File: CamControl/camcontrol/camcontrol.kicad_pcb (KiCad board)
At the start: 2 copper layers, 35 x 35 mm, 74 parts, among them J2 USB_B_Micro, J3 Conn_01x03, J4 Conn_01x02, J5 Conn_01x02, J6 Conn_01x02, J7 Conn_01x03, J8 Conn_01x04, Q2 AO3401A, Q3 AO3401A, U1 E22-900MM22S, U2 TPS1HC30BQPWPRQ1, U3 TPS63060DSCR, U4 XC6206P332MR, U5 W25Q128JVS, U6 RP2040, U7 TPS1HC30BQPWPRQ1, X1 SX1M12.000M10F30TNN

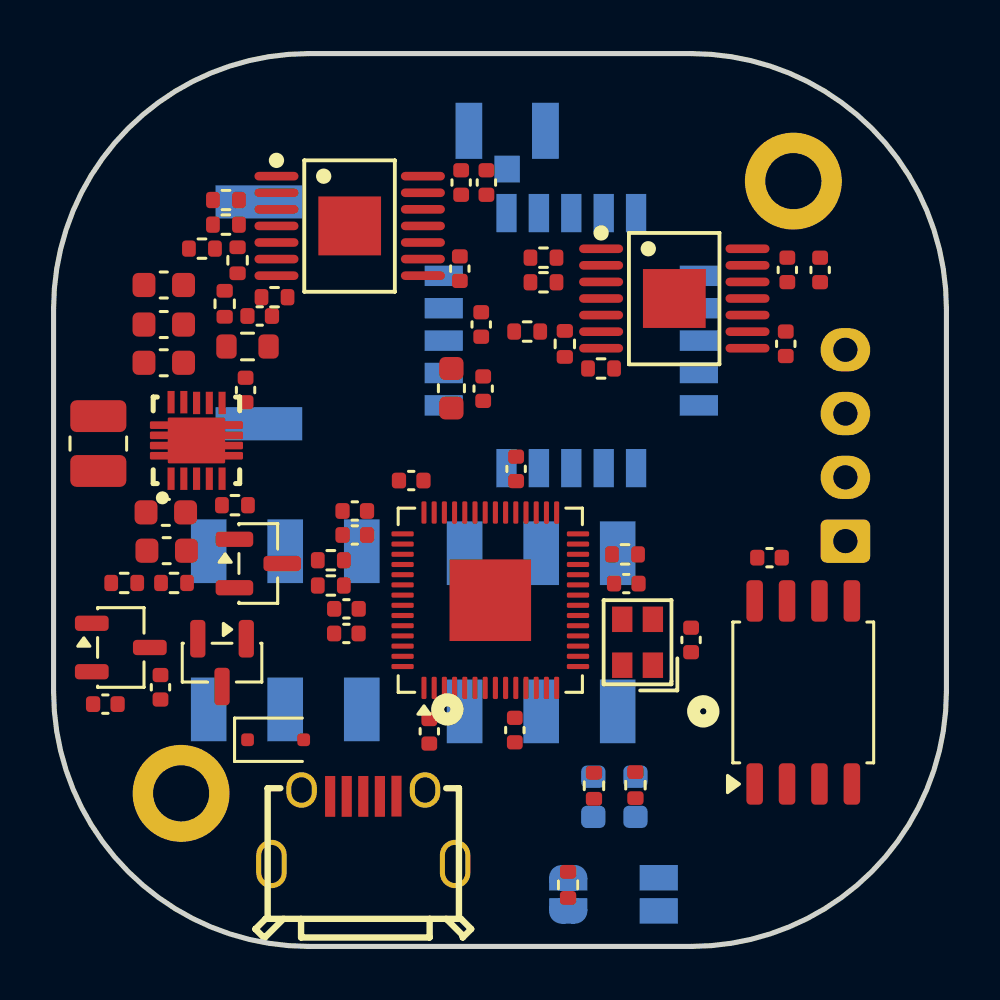
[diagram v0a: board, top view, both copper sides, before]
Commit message: first routing pass
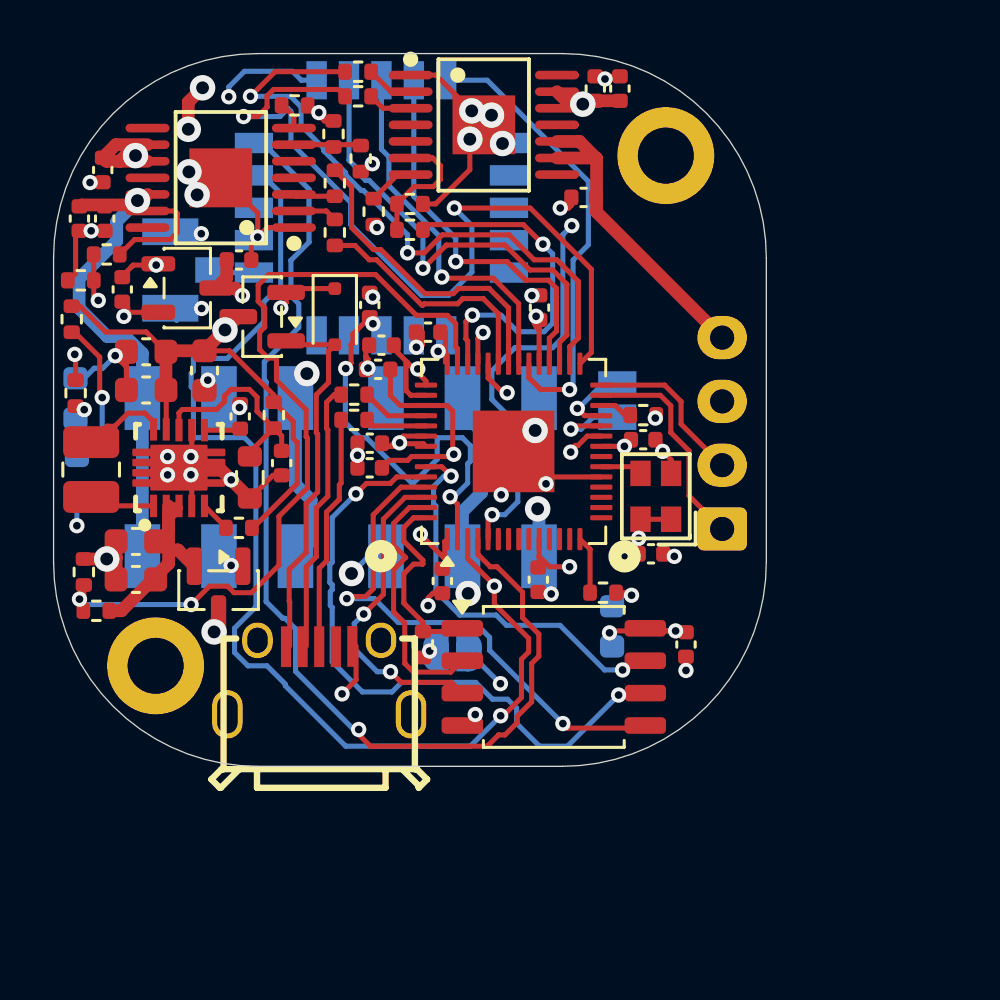
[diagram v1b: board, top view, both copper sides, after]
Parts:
- removed C2: 10n, Capacitor_SMD:C_0402_1005Metric
- removed C3: 10u, Capacitor_SMD:C_0603_1608Metric
- removed J4: Conn_01x02, SamacSys_Parts:PKMCS0909E4000R1
- added D2: LED, LED_SMD:LED_0603_1608Metric, B.Cu at (159.9, 136.4)
- added R22: 1k, Resistor_SMD:R_0402_1005Metric, F.Cu at (159.7, 130.2)
- added R23: 27k, Resistor_SMD:R_0402_1005Metric, F.Cu at (161.0, 127.7)
- added R24: 51k, Resistor_SMD:R_0402_1005Metric, F.Cu at (160.0, 128.7)
- moved D1 26.9 mm to (159.8, 133.4), turned to -90 degrees
- moved R1 26.8 mm to (159.8, 133.1), turned to 90 degrees
- moved J5 19.4 mm to (181.1, 133.4)
- moved C5 17.0 mm to (166.2, 127.9), turned to 0 degrees
- moved D4 16.7 mm to (170.0, 130.1), turned to -90 degrees
- moved C6 16.3 mm to (161.6, 129.1), turned to 90 degrees
- moved C29 16.0 mm to (160.0, 126.3), turned to -90 degrees
- moved C30 14.5 mm to (160.9, 124.4)
- moved U4 14.3 mm to (164.2, 129.0)
- moved C28 14.0 mm to (161.0, 126.3), turned to -90 degrees
- moved Q3 13.7 mm to (167.1, 130.1), turned to 180 degrees
- moved AE1 13.3 mm to (164.3, 128.3), turned to 90 degrees
- moved R3 11.0 mm to (173.4, 143.0), turned to -90 degrees
- moved R12 10.8 mm to (171.5, 126.0), turned to -90 degrees
- moved C26 10.6 mm to (181.2, 121.2)
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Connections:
- Q3 pad 3: /BATT POSTSW -> +5V
- U6 pad 11: /LEDINDICATION -> unconnected-(U6-GPIO8-Pad11)
- U6 pad 14: unconnected-(U6-GPIO11-Pad14) -> /LEDINDICATION
- U6 pad 2: unconnected-(U6-GPIO0-Pad2) -> /SX RST
- U6 pad 27: /MISO -> /CAM RX
- U6 pad 28: unconnected-(U6-GPIO17-Pad28) -> /CAM TX
- U6 pad 29: /SCLK -> /CAM DIAG EN
- U6 pad 3: unconnected-(U6-GPIO1-Pad3) -> /TXEN
- U6 pad 30: /MOSI -> /CAM EN
- U6 pad 31: unconnected-(U6-GPIO20-Pad31) -> /MISO
- U6 pad 32: unconnected-(U6-GPIO21-Pad32) -> /SX CS
- U6 pad 34: unconnected-(U6-GPIO22-Pad34) -> /SCLK
- U6 pad 35: unconnected-(U6-GPIO23-Pad35) -> /MOSI
- U6 pad 36: unconnected-(U6-GPIO24-Pad36) -> /VID DIAG EN
- U6 pad 37: unconnected-(U6-GPIO25-Pad37) -> /VID EN
- U6 pad 4: unconnected-(U6-GPIO2-Pad4) -> /RXEN
- U6 pad 5: unconnected-(U6-GPIO3-Pad5) -> /BUSY
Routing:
- net GND: track 0.00 -> 59.5 mm, vias 0 -> 45
- net +5V: track 0.00 -> 49.4 mm, vias 0 -> 4
- net /TXEN: track 0.00 -> 45.0 mm, vias 0 -> 2
- net /RXEN: track 0.00 -> 42.4 mm, vias 0 -> 1
- net /BUSY: track 0.00 -> 40.5 mm, vias 0 -> 3
- net /TX BATT SENSE : track 0.00 -> 32.9 mm, vias 0 -> 2
- net /CAM BATT SENSE : track 0.00 -> 32.7 mm, vias 0 -> 2
- net /CAM DIAG EN: track 0.00 -> 31.6 mm, vias 0 -> 2
- net +3V3: track 0.00 -> 27.7 mm, vias 0 -> 13
- net /VIDPWR: track 0.00 -> 25.7 mm, vias 0 -> 2
- net /CAM EN: track 0.00 -> 24.9 mm, vias 0 -> 2
- net /QSPI_SCLK: track 0.00 -> 24.2 mm, vias 0 -> 2
- net +12V: track 0.00 -> 23.7 mm, vias 0 -> 1
- net +BATT: track 0.00 -> 21.7 mm, vias 0 -> 2
- net /QSPI_SDO: track 0.00 -> 20.7 mm, vias 0 -> 2
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- added copper zone on In2.Cu, net +3V3
- added copper zone on In1.Cu, net GND
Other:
- board size 35 x 35 mm -> 27.9 x 27.9 mm
- copper layers 2 -> 4
